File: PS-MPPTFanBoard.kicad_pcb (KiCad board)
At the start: 2 copper layers, 100 x 49 mm, 139 parts, among them IC1 TCAN3413DR, IC2 LM74502DDFR, IC3 TCAN3413DR, J1 Fan 1, 2, J11 USB_C_Receptacle_USB2.0_16P, J2 Fan 3, 4, J5 SWD_Header, J6 SWD, Q1 PSMN012-100YS, Q2 PSMN012-100YS, SW1 Reset, SW2 SW_SPDT, U1 EMC2305-1-AP-TR, U2 STM32G473CETx, U3 MCP1826S, U4 LMR51635XDDCR, U5 TPS2117DRLR, Y1 Crystal

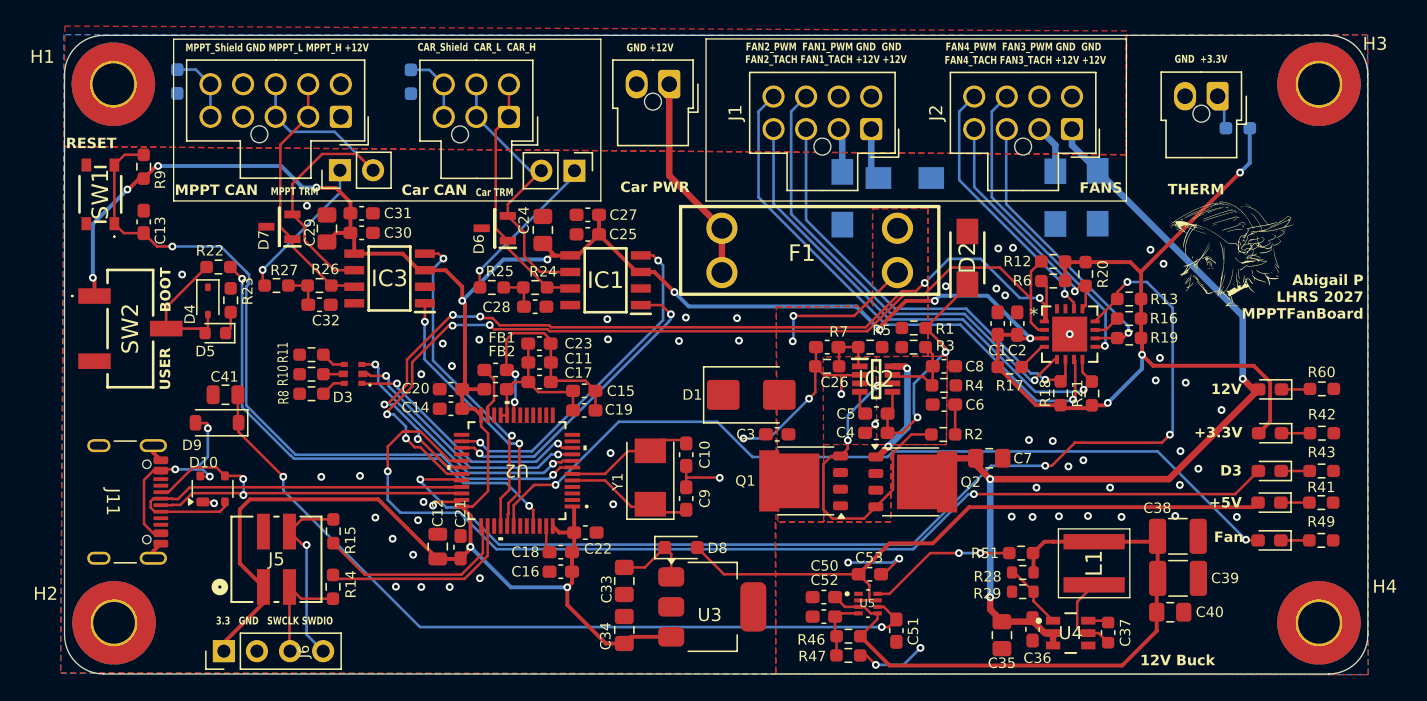
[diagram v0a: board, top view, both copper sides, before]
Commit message: bom and gerber
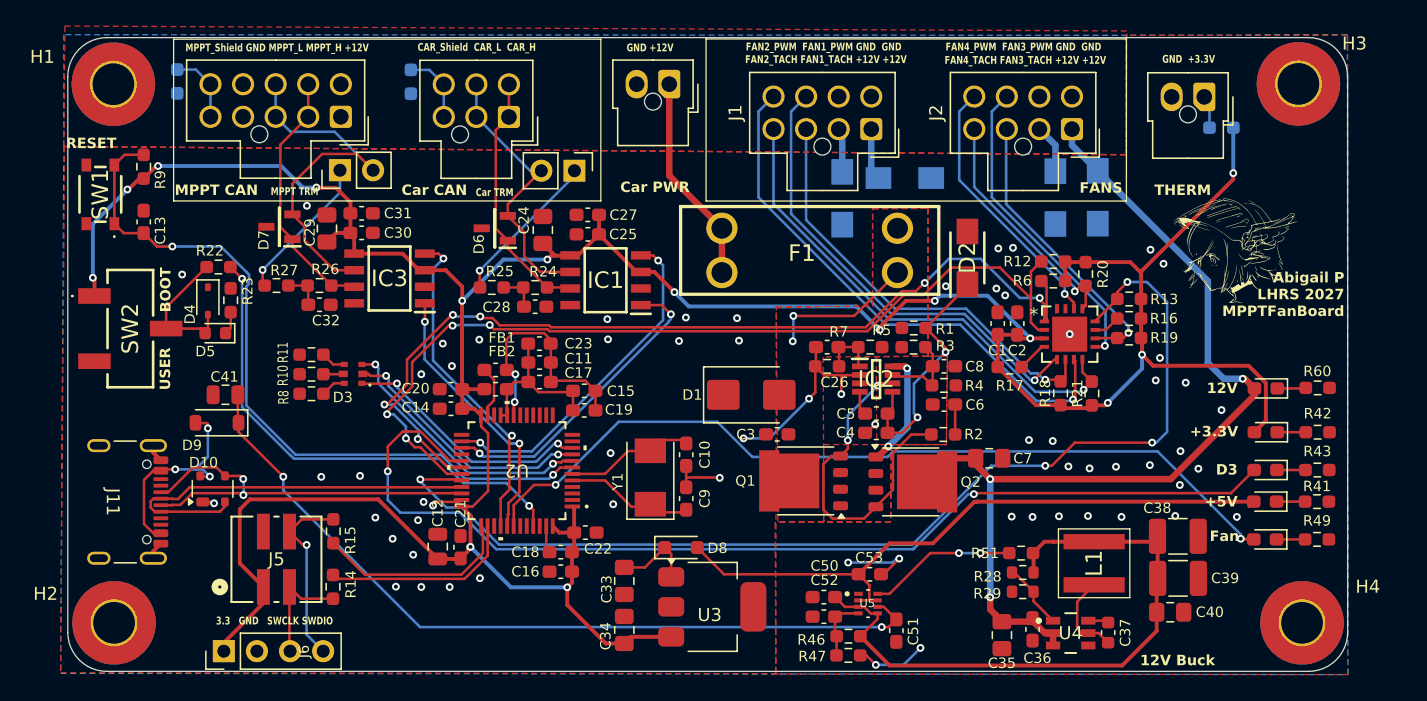
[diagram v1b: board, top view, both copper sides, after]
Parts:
- moved H3 1.58 mm to (173.2, 57.0)
- moved LOGO4 1.50 mm to (170.2, 76.5)
- moved H4 1.30 mm to (173.4, 98.3)
- moved R45 1.26 mm to (167.3, 60.3)
- moved THERM 1.03 mm to (163.4, 58.0)
- moved G*** 0.38 mm to (168.3, 69.6)
- moved R49 0.33 mm to (174.6, 91.9)
- moved R41 0.33 mm to (174.6, 89.0)
- moved +3.3V 0.33 mm to (170.7, 83.7)
- moved 12V 0.33 mm to (170.7, 80.3)
- moved D3 0.33 mm to (170.7, 86.6)
- moved Fan 0.33 mm to (170.6, 91.9)
- moved R42 0.33 mm to (174.7, 83.7)
- moved R43 0.33 mm to (174.6, 86.6)
- moved R60 0.33 mm to (174.7, 80.3)
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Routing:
- net +3.3V: track 248.2 -> 247.1 mm
- net /FAN_CHIP: track 65.5 -> 66.2 mm
- net /~{SMBALERT}: track 84.5 -> 83.9 mm
- net +12V: track 84.8 -> 85.3 mm
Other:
- board size 100 x 49 mm -> 98.2 x 48.6 mm
